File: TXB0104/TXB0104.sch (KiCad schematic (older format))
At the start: 6 parts, among them J1 Conn_01x06, J2 Conn_01x06, U1 TXB0104PW

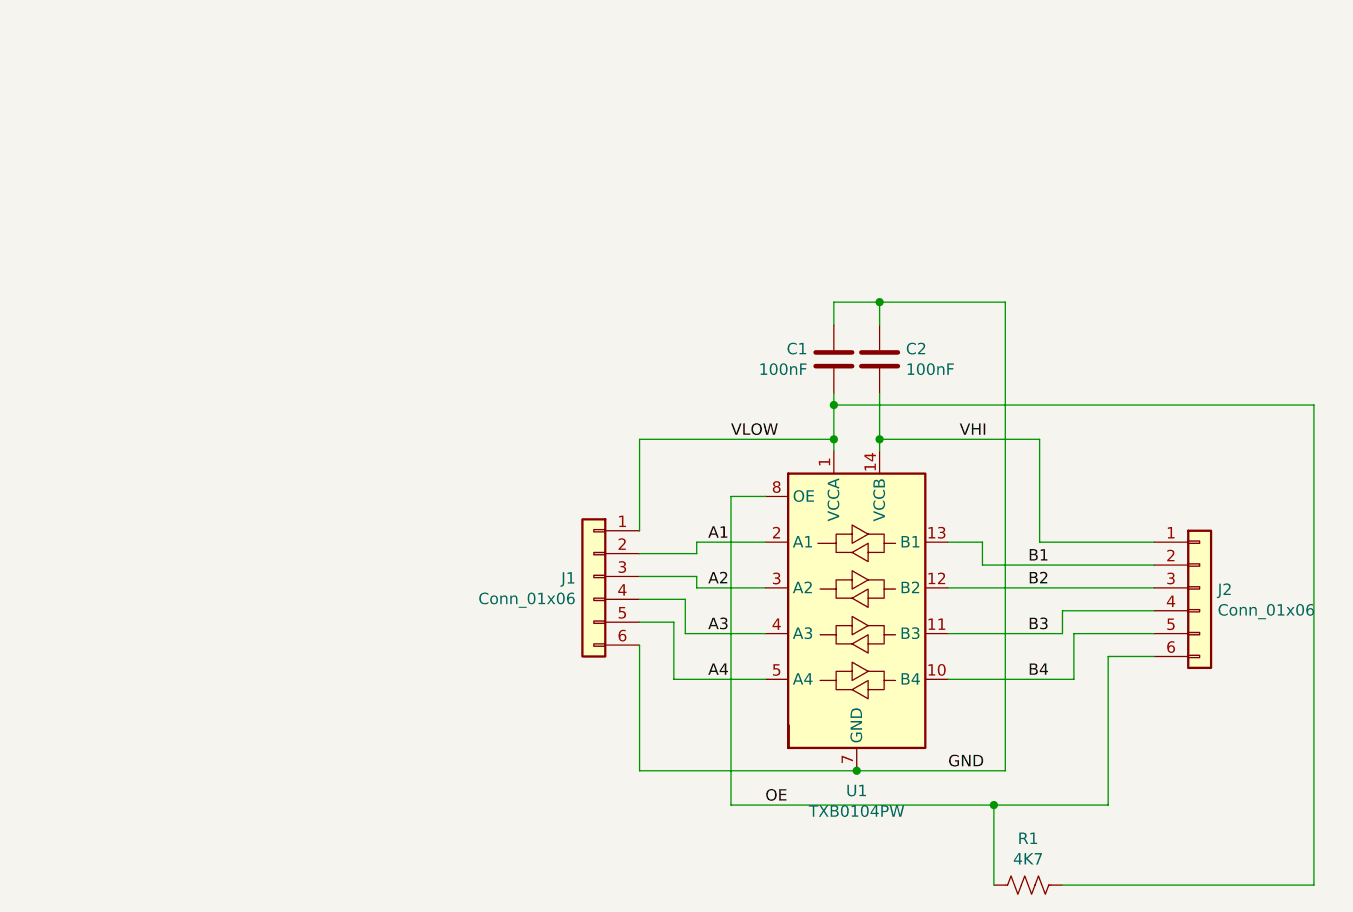
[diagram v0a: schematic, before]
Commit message: Part Numbers Added
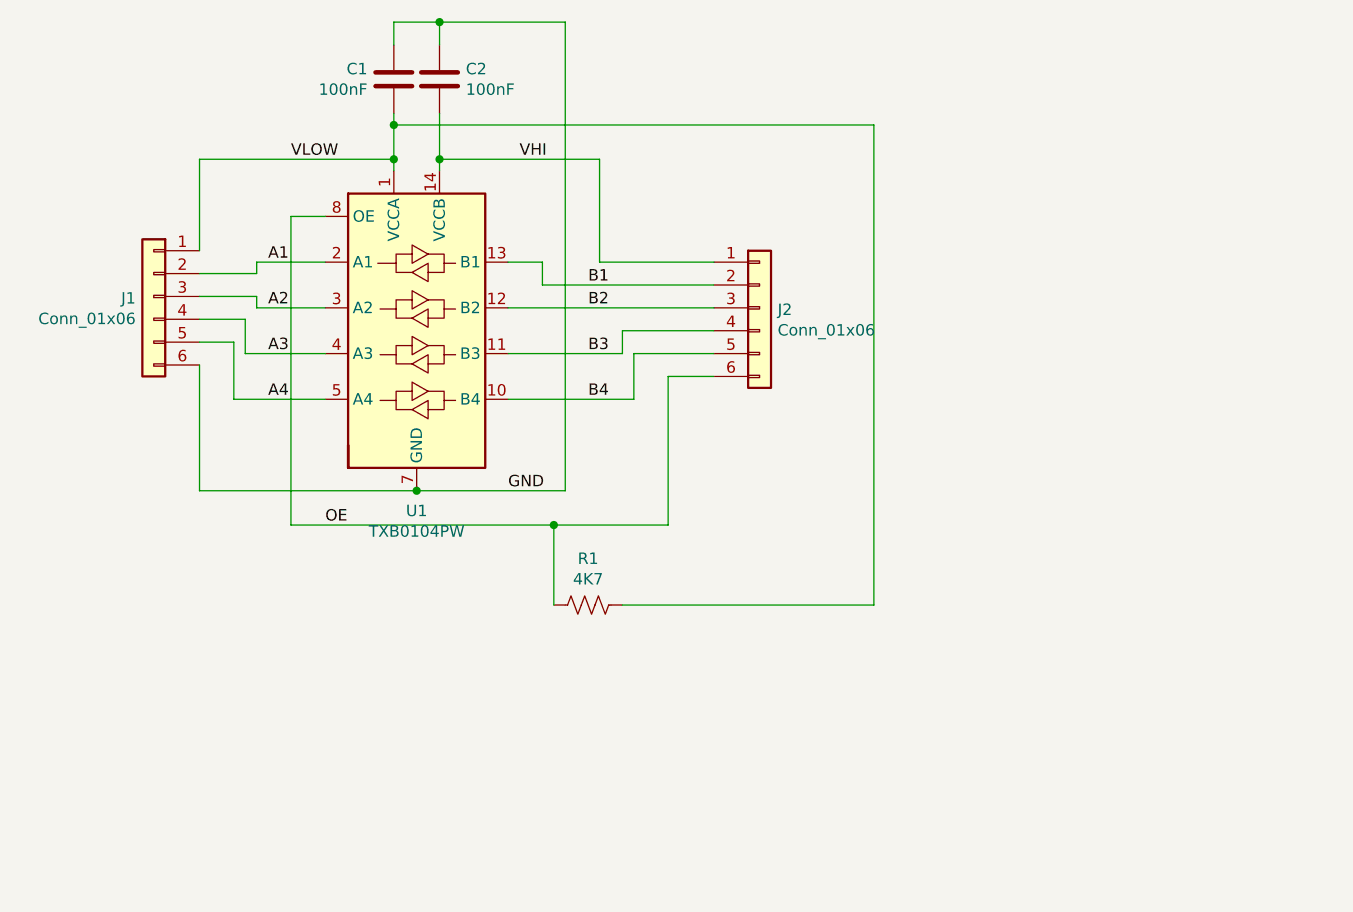
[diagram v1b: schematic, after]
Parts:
- C1, C2: Part (none) -> C38141
- R1: Part (none) -> C99782
- U1: Part (none) -> C60708
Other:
- moved on the sheet: C1, C2, J1, J2, R1, U1
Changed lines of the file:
@@
 EELAYER 29 0
 EELAYER END
-$Descr A4 11693 8268
+$Descr User 8268 5807
 encoding utf-8
 Sheet 1 1
-Title ""
-Date ""
-Rev ""
-Comp ""
-Comment1 ""
-Comment2 ""
-Comment3 ""
+Title "4 Channel Bi-Directional Level Shifter"
+Date "2019-09-16"
+Rev "1"
+Comp "SirBoard"
+Comment1 "www.SirBoard.com"
+Comment2 "TXB0104"
+Comment3 "SirLevel"
 Comment4 ""
 $EndDescr
@@
 L Device:C C2
 U 1 1 5D2E53A3
-P 5600 2600
-F 0 "C2" H 5715 2645 50  0000 L CNN
-F 1 "100nF" H 5715 2555 50  0000 L CNN
-F 2 "Capacitor_SMD:C_0805_2012Metric_Pad1.15x1.40mm_HandSolder" H 5638 2450 50  0001 C CNN
-F 3 "~" H 5600 2600 50  0001 C CNN
-	1    5600 2600
+P 3675 1375
+F 0 "C2" H 3790 1420 50  0000 L CNN
+F 1 "100nF" H 3790 1330 50  0000 L CNN
+F 2 "Capacitor_SMD:C_0805_2012Metric_Pad1.15x1.40mm_HandSolder" H 3713 1225 50  0001 C CNN
+F 3 "~" H 3675 1375 50  0001 C CNN
+F 4 "C38141" H 3675 1375 50  0001 C CNN "Part"
+	1    3675 1375
 	1    0    0    -1
 $EndComp
@@
 L Device:C C1
 U 1 1 5D2E61B4
-P 5400 2600
-F 0 "C1" H 5515 2645 50  0000 L CNN
-F 1 "100nF" H 5515 2555 50  0000 L CNN
-F 2 "Capacitor_SMD:C_0805_2012Metric_Pad1.15x1.40mm_HandSolder" H 5438 2450 50  0001 C CNN
-F 3 "~" H 5400 2600 50  0001 C CNN
-	1    5400 2600
+P 3475 1375
+F 0 "C1" H 3590 1420 50  0000 L CNN
+F 1 "100nF" H 3590 1330 50  0000 L CNN
+F 2 "Capacitor_SMD:C_0805_2012Metric_Pad1.15x1.40mm_HandSolder" H 3513 1225 50  0001 C CNN
+F 3 "~" H 3475 1375 50  0001 C CNN
+F 4 "C38141" H 3475 1375 50  0001 C CNN "Part"
+	1    3475 1375
 	-1   0    0    -1
 $EndComp
 Wire Wire Line
-	5400 3000 5400 2950
-Wire Wire Line
-	5600 3000 5600 2950
-Wire Wire Line
-	5400 2450 5400 2350
-Wire Wire Line
-	5400 2350 5600 2350
-Wire Wire Line
-	5600 2350 5600 2450
-Wire Wire Line
-	6150 4400 6150 2350
-Wire Wire Line
-	6150 2350 5600 2350
-Connection ~ 5600 2350
+	3475 1775 3475 1725
+Wire Wire Line
+	3675 1775 3675 1725
+Wire Wire Line
+	3475 1225 3475 1125
+Wire Wire Line
+	3475 1125 3675 1125
+Wire Wire Line
+	3675 1125 3675 1225
+Wire Wire Line
+	4225 3175 4225 1125
+Wire Wire Line
+	4225 1125 3675 1125
+Connection ~ 3675 1125
 $Comp
 L Connector_Generic:Conn_01x06 J2
 U 1 1 5D2E7899
-P 7000 3600
-F 0 "J2" H 7079 3592 50  0000 L CNN
-F 1 "Conn_01x06" H 7079 3502 50  0000 L CNN
-F 2 "Connector_PinHeader_2.54mm:PinHeader_1x06_P2.54mm_Vertical" H 7000 3600 50  0001 C CNN
-F 3 "~" H 7000 3600 50  0001 C CNN
-	1    7000 3600
+P 5075 2375
+F 0 "J2" H 5154 2367 50  0000 L CNN
+F 1 "Conn_01x06" H 5154 2277 50  0000 L CNN
+F 2 "Connector_PinHeader_2.54mm:PinHeader_1x06_P2.54mm_Vertical" H 5075 2375 50  0001 C CNN
+F 3 "~" H 5075 2375 50  0001 C CNN
+	1    5075 2375
 	1    0    0    -1
 $EndComp
@@
 L Connector_Generic:Conn_01x06 J1
 U 1 1 5D2E8423
-P 4350 3550
-F 0 "J1" H 4429 3542 50  0000 L CNN
-F 1 "Conn_01x06" H 4429 3452 50  0000 L CNN
-F 2 "Connector_PinHeader_2.54mm:PinHeader_1x06_P2.54mm_Vertical" H 4350 3550 50  0001 C CNN
-F 3 "~" H 4350 3550 50  0001 C CNN
-	1    4350 3550
+P 2425 2325
+F 0 "J1" H 2504 2317 50  0000 L CNN
+F 1 "Conn_01x06" H 2504 2227 50  0000 L CNN
+F 2 "Connector_PinHeader_2.54mm:PinHeader_1x06_P2.54mm_Vertical" H 2425 2325 50  0001 C CNN
+F 3 "~" H 2425 2325 50  0001 C CNN
+	1    2425 2325
 	-1   0    0    -1
 $EndComp
 Wire Wire Line
-	5400 2950 4550 2950
-Wire Wire Line
-	4550 2950 4550 3350
-Connection ~ 5400 2950
-Wire Wire Line
-	5400 2950 5400 2800
-Wire Wire Line
-	4550 3450 4800 3450
-Wire Wire Line
-	4800 3450 4800 3400
-Wire Wire Line
-	4800 3400 5100 3400
-Wire Wire Line
-	4550 3550 4800 3550
-Wire Wire Line
-	4800 3550 4800 3600
-Wire Wire Line
-	4800 3600 5100 3600
-Wire Wire Line
-	4550 3650 4750 3650
-Wire Wire Line
-	4750 3650 4750 3800
-Wire Wire Line
-	4750 3800 5100 3800
-Wire Wire Line
-	4550 3750 4700 3750
-Wire Wire Line
-	4700 3750 4700 4000
-Wire Wire Line
-	4700 4000 5100 4000
-Wire Wire Line
-	5100 3200 4950 3200
-Wire Wire Line
-	4950 3200 4950 4550
-Wire Wire Line
-	4950 4550 6100 4550
-Wire Wire Line
-	6600 4550 6600 3900
-Wire Wire Line
-	6600 3900 6800 3900
-Wire Wire Line
-	5900 4000 6450 4000
-Wire Wire Line
-	6450 4000 6450 3800
-Wire Wire Line
-	6450 3800 6800 3800
-Wire Wire Line
-	5900 3800 6400 3800
-Wire Wire Line
-	6400 3800 6400 3700
-Wire Wire Line
-	6400 3700 6800 3700
-Wire Wire Line
-	5900 3600 6800 3600
-Wire Wire Line
-	6800 3500 6050 3500
-Wire Wire Line
-	6050 3500 6050 3400
-Wire Wire Line
-	6050 3400 5900 3400
-Wire Wire Line
-	6800 3400 6300 3400
-Wire Wire Line
-	6300 3400 6300 2950
-Wire Wire Line
-	6300 2950 5600 2950
-Connection ~ 5600 2950
-Wire Wire Line
-	5600 2950 5600 2750
-Text Label 5900 4400 0    50   ~ 0
+	3475 1725 2625 1725
+Wire Wire Line
+	2625 1725 2625 2125
+Connection ~ 3475 1725
+Wire Wire Line
+	3475 1725 3475 1575
+Wire Wire Line
+	2625 2225 2875 2225
+Wire Wire Line
+	2875 2225 2875 2175
+Wire Wire Line
+	2875 2175 3175 2175
+Wire Wire Line
+	2625 2325 2875 2325
+Wire Wire Line
+	2875 2325 2875 2375
+Wire Wire Line
+	2875 2375 3175 2375
+Wire Wire Line
+	2625 2425 2825 2425
+Wire Wire Line
+	2825 2425 2825 2575
+Wire Wire Line
+	2825 2575 3175 2575
+Wire Wire Line
+	2625 2525 2775 2525
+Wire Wire Line
+	2775 2525 2775 2775
+Wire Wire Line
+	2775 2775 3175 2775
+Wire Wire Line
+	3175 1975 3025 1975
+Wire Wire Line
+	3025 1975 3025 3325
+Wire Wire Line
+	3025 3325 4175 3325
+Wire Wire Line
+	4675 3325 4675 2675
+Wire Wire Line
+	4675 2675 4875 2675
+Wire Wire Line
+	3975 2775 4525 2775
+Wire Wire Line
+	4525 2775 4525 2575
+Wire Wire Line
+	4525 2575 4875 2575
+Wire Wire Line
+	3975 2575 4475 2575
+Wire Wire Line
+	4475 2575 4475 2475
+Wire Wire Line
+	4475 2475 4875 2475
+Wire Wire Line
+	3975 2375 4875 2375
+Wire Wire Line
+	4875 2275 4125 2275
+Wire Wire Line
+	4125 2275 4125 2175
+Wire Wire Line
+	4125 2175 3975 2175
+Wire Wire Line
+	4875 2175 4375 2175
+Wire Wire Line
+	4375 2175 4375 1725
+Wire Wire Line
+	4375 1725 3675 1725
+Connection ~ 3675 1725
+Wire Wire Line
+	3675 1725 3675 1525
+Text Label 3975 3175 0    50   ~ 0
 GND
-Text Label 5950 2950 0    50   ~ 0
+Text Label 4025 1725 0    50   ~ 0
 VHI
-Text Label 4950 2950 0    50   ~ 0
+Text Label 3025 1725 0    50   ~ 0
 VLOW
-Text Label 5100 4550 0    50   ~ 0
+Text Label 3175 3325 0    50   ~ 0
 OE
-Text Label 4850 3400 0    50   ~ 0
+Text Label 2925 2175 0    50   ~ 0
 A1
-Text Label 4850 3600 0    50   ~ 0
+Text Label 2925 2375 0    50   ~ 0
 A2
-Text Label 4850 3800 0    50   ~ 0
+Text Label 2925 2575 0    50   ~ 0
 A3
-Text Label 4850 4000 0    50   ~ 0
+Text Label 2925 2775 0    50   ~ 0
 A4
-Text Label 6250 3500 0    50   ~ 0
+Text Label 4325 2275 0    50   ~ 0
 B1
-Text Label 6250 3600 0    50   ~ 0
+Text Label 4325 2375 0    50   ~ 0
 B2
-Text Label 6250 3800 0    50   ~ 0
+Text Label 4325 2575 0    50   ~ 0
 B3
-Text Label 6250 4000 0    50   ~ 0
+Text Label 4325 2775 0    50   ~ 0
 B4
 $Comp
 L Device:R_US R1
 U 1 1 5D2FAE97
-P 6250 4900
-F 0 "R1" V 6047 4900 50  0000 C CNN
-F 1 "4K7" V 6137 4900 50  0000 C CNN
-F 2 "Resistor_SMD:R_0805_2012Metric_Pad1.15x1.40mm_HandSolder" V 6290 4890 50  0001 C CNN
-F 3 "~" H 6250 4900 50  0001 C CNN
-	1    6250 4900
+P 4325 3675
+F 0 "R1" V 4122 3675 50  0000 C CNN
+F 1 "4K7" V 4212 3675 50  0000 C CNN
+F 2 "Resistor_SMD:R_0805_2012Metric_Pad1.15x1.40mm_HandSolder" V 4365 3665 50  0001 C CNN
+F 3 "~" H 4325 3675 50  0001 C CNN
+F 4 "C99782" V 4325 3675 50  0001 C CNN "Part"
+	1    4325 3675
 	0    1    1    0
 $EndComp
 Wire Wire Line
-	6100 4550 6100 4900
-Wire Wire Line
-	6100 4550 6600 4550
-Connection ~ 6100 4550
-Wire Wire Line
-	6400 4900 7500 4900
-Wire Wire Line
-	7500 4900 7500 2800
-Wire Wire Line
-	7500 2800 5400 2800
-Connection ~ 5400 2800
-Wire Wire Line
-	5400 2800 5400 2750
+	4175 3325 4175 3675
+Wire Wire Line
+	4175 3325 4675 3325
+Connection ~ 4175 3325
+Wire Wire Line
+	4475 3675 5575 3675
+Wire Wire Line
+	5575 3675 5575 1575
+Wire Wire Line
+	5575 1575 3475 1575
+Connection ~ 3475 1575
+Wire Wire Line
+	3475 1575 3475 1525
 $Comp
 L Logic_LevelTranslator:TXB0104PW U1
 U 1 1 5D8F47CC
-P 5500 3700
-F 0 "U1" H 5500 2912 50  0000 C CNN
-F 1 "TXB0104PW" H 5500 2822 50  0000 C CNN
-F 2 "Package_SO:TSSOP-14_4.4x5mm_P0.65mm" H 5500 2950 50  0001 C CNN
-F 3 "http://www.ti.com/lit/ds/symlink/txb0104.pdf" H 5610 3795 50  0001 C CNN
-	1    5500 3700
+P 3575 2475
+F 0 "U1" H 3575 1687 50  0000 C CNN
+F 1 "TXB0104PW" H 3575 1597 50  0000 C CNN
+F 2 "Package_SO:TSSOP-14_4.4x5mm_P0.65mm" H 3575 1725 50  0001 C CNN
+F 3 "http://www.ti.com/lit/ds/symlink/txb0104.pdf" H 3685 2570 50  0001 C CNN
+F 4 "C60708" H 3575 2475 50  0001 C CNN "Part"
+	1    3575 2475
 	1    0    0    -1
 $EndComp
 Wire Wire Line
-	4550 4400 5500 4400
-Connection ~ 5500 4400
-Wire Wire Line
-	5500 4400 6150 4400
-Wire Wire Line
-	4550 3850 4550 4400
+	2625 3175 3575 3175
+Connection ~ 3575 3175
+Wire Wire Line
+	3575 3175 4225 3175
+Wire Wire Line
+	2625 2625 2625 3175
 $EndSCHEMATC
